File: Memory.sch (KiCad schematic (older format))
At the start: 2 parts, among them U2 27C256, U3 IS61C256AH

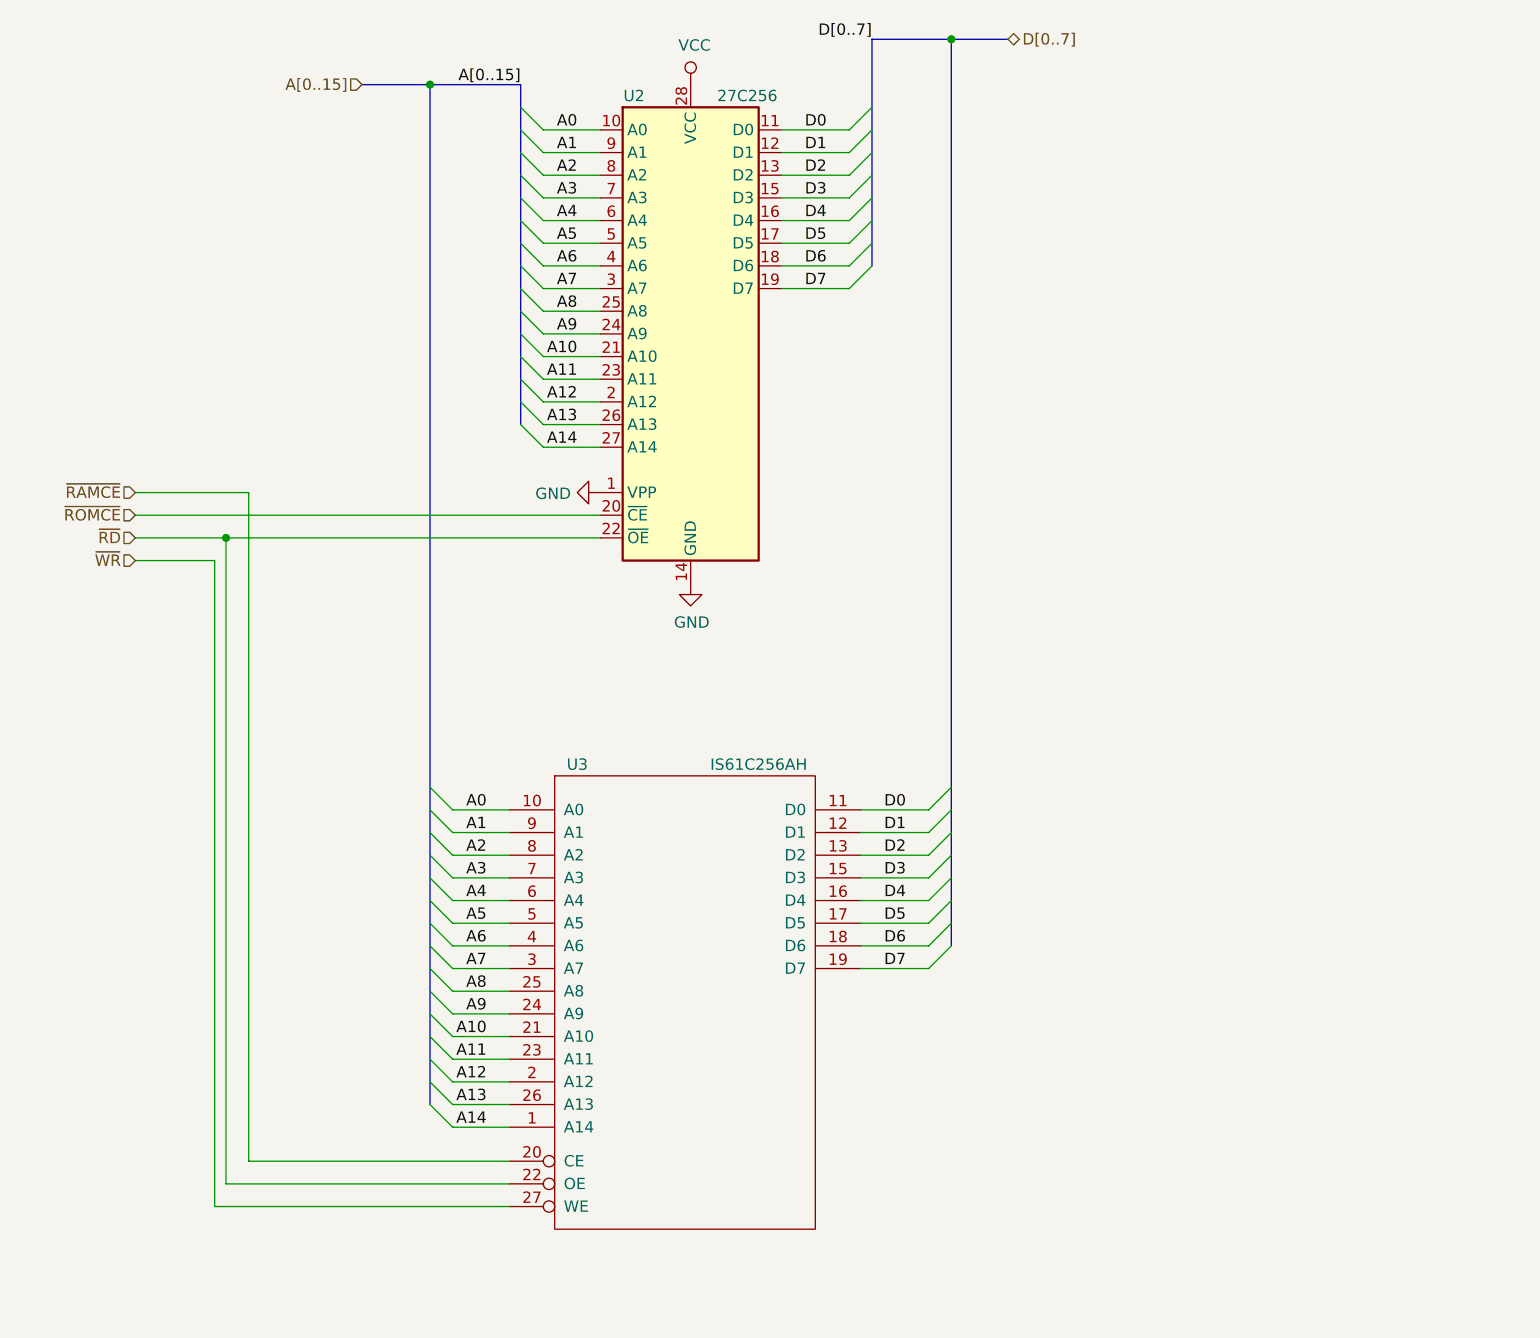
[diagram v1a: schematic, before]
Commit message: RevC
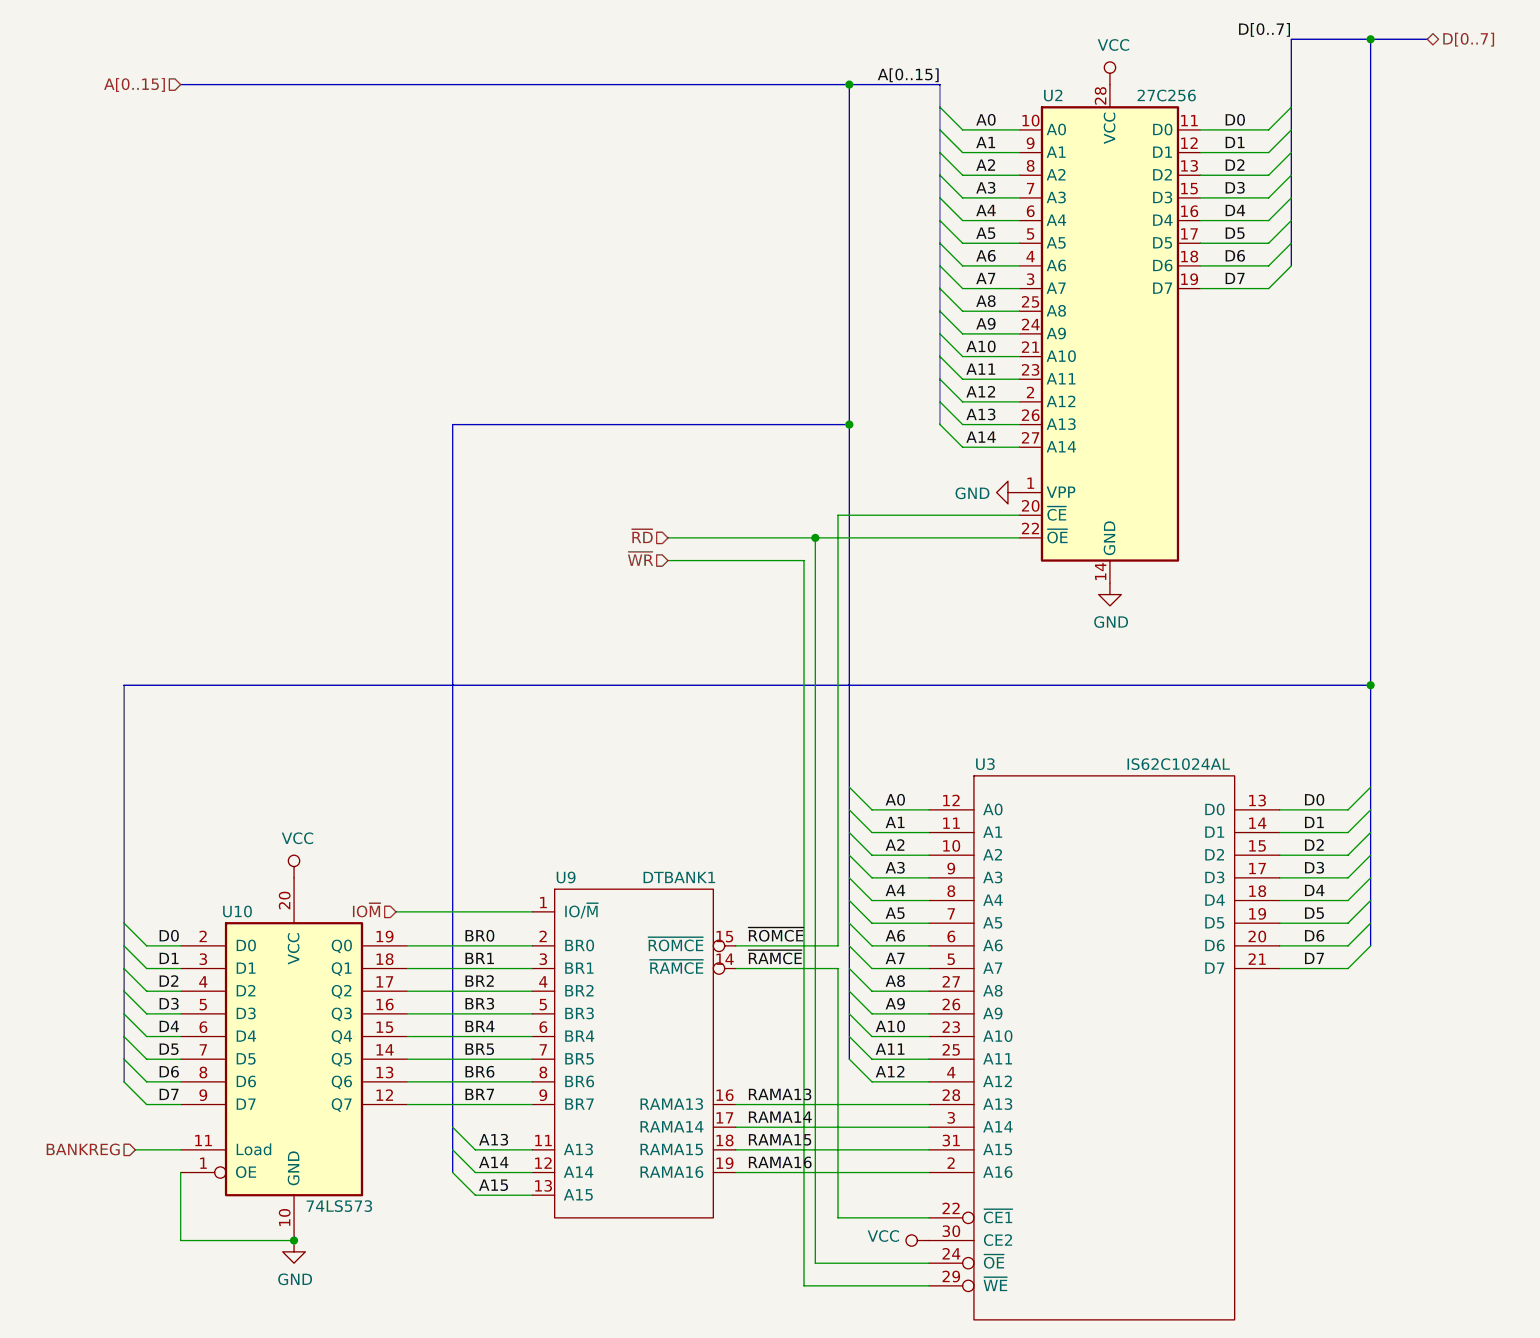
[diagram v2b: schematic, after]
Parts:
- removed U3: IS61C256AH, Package_DIP:DIP-28_W7.62mm, symbol 8085:IS61C256AH
- added U10: 74LS573, Package_DIP:DIP-20_W7.62mm, symbol 74xx:74LS573
- added U3: IS62C1024AL, 8085:SOIC-32W_14x21mm_P1.27mm, symbol 8085:IS62C1024AL
- added U9: DTBANK1, Package_DIP:DIP-20_W7.62mm, symbol 8085:DTBANK1
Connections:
- net A0: now also U3.12 (A0)
- net A1: now also U3.11 (A1)
- net A10: now also U3.23 (A10)
- net A11: now also U3.25 (A11)
- net A12: now also U3.4 (A12)
- net A13: now also U9.11 (A13)
- net A14: now also U9.12 (A14)
- net A2: now also U3.10 (A2)
- net A3: now also U3.9 (A3)
- net A4: now also U3.8 (A4)
- net A5: now also U3.7 (A5)
- net A6: now also U3.6 (A6)
- net A7: now also U3.5 (A7)
- net A8: now also U3.27 (A8)
- net A9: now also U3.26 (A9)
- net D0: now also U10.2 (D0), U3.13 (D0)
- net D1: now also U10.3 (D1), U3.14 (D1)
- net D2: now also U10.4 (D2), U3.15 (D2)
- net D3: now also U10.5 (D3), U3.17 (D3)
- net D4: now also U10.6 (D4), U3.18 (D4)
- net D5: now also U10.7 (D5), U3.19 (D5)
- net D6: now also U10.8 (D6), U3.20 (D6)
- net D7: now also U10.9 (D7), U3.21 (D7)
- net GND: now also U10.1 (OE), U10.10 (GND), U3.16 (GND), U9.10 (GND)
- net VCC: now also U10.20 (VCC), U3.30 (CE2), U3.32 (VCC), U9.20 (VCC)
- net ~RAMCE: now also U3.22 (~CE1), U9.14 (~RAMCE)
- net ~RD: now also U3.24 (~OE)
- net ~ROMCE: now also U9.15 (~ROMCE)
- net ~WR: now also U3.29 (~WE)
- new net A15: U9.13 (A15)
- new net BANKREG: U10.11 (Load)
- new net BR0: U10.19 (Q0), U9.2 (BR0)
- new net BR1: U10.18 (Q1), U9.3 (BR1)
- new net BR2: U10.17 (Q2), U9.4 (BR2)
- new net BR3: U10.16 (Q3), U9.5 (BR3)
- new net BR4: U10.15 (Q4), U9.6 (BR4)
- new net BR5: U10.14 (Q5), U9.7 (BR5)
- new net BR6: U10.13 (Q6), U9.8 (BR6)
- new net BR7: U10.12 (Q7), U9.9 (BR7)
- new net IO~M: U9.1 (IO/~M)
- new net RAMA13: U3.28 (A13), U9.16 (RAMA13)
- new net RAMA14: U3.3 (A14), U9.17 (RAMA14)
- new net RAMA15: U3.31 (A15), U9.18 (RAMA15)
- new net RAMA16: U3.2 (A16), U9.19 (RAMA16)
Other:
- moved on the sheet: U2
